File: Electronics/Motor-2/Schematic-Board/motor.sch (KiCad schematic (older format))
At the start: 42 parts, among them J1 CONN_02X05, J11 V, J12 U, J13 W, J2 RS485, J3 RS485, J4 CONN_01X06, J6 12, J9 GND, Q1 PSMN3R3-40YS, Q2 PSMN3R3-40YS, Q3 PSMN3R3-40YS, Q4 PSMN3R3-40YS, Q5 PSMN3R3-40YS, Q6 PSMN3R3-40YS, U1 STSPIN32F0, U2 LTC2876, U3 MA700, Y1 8Mhz

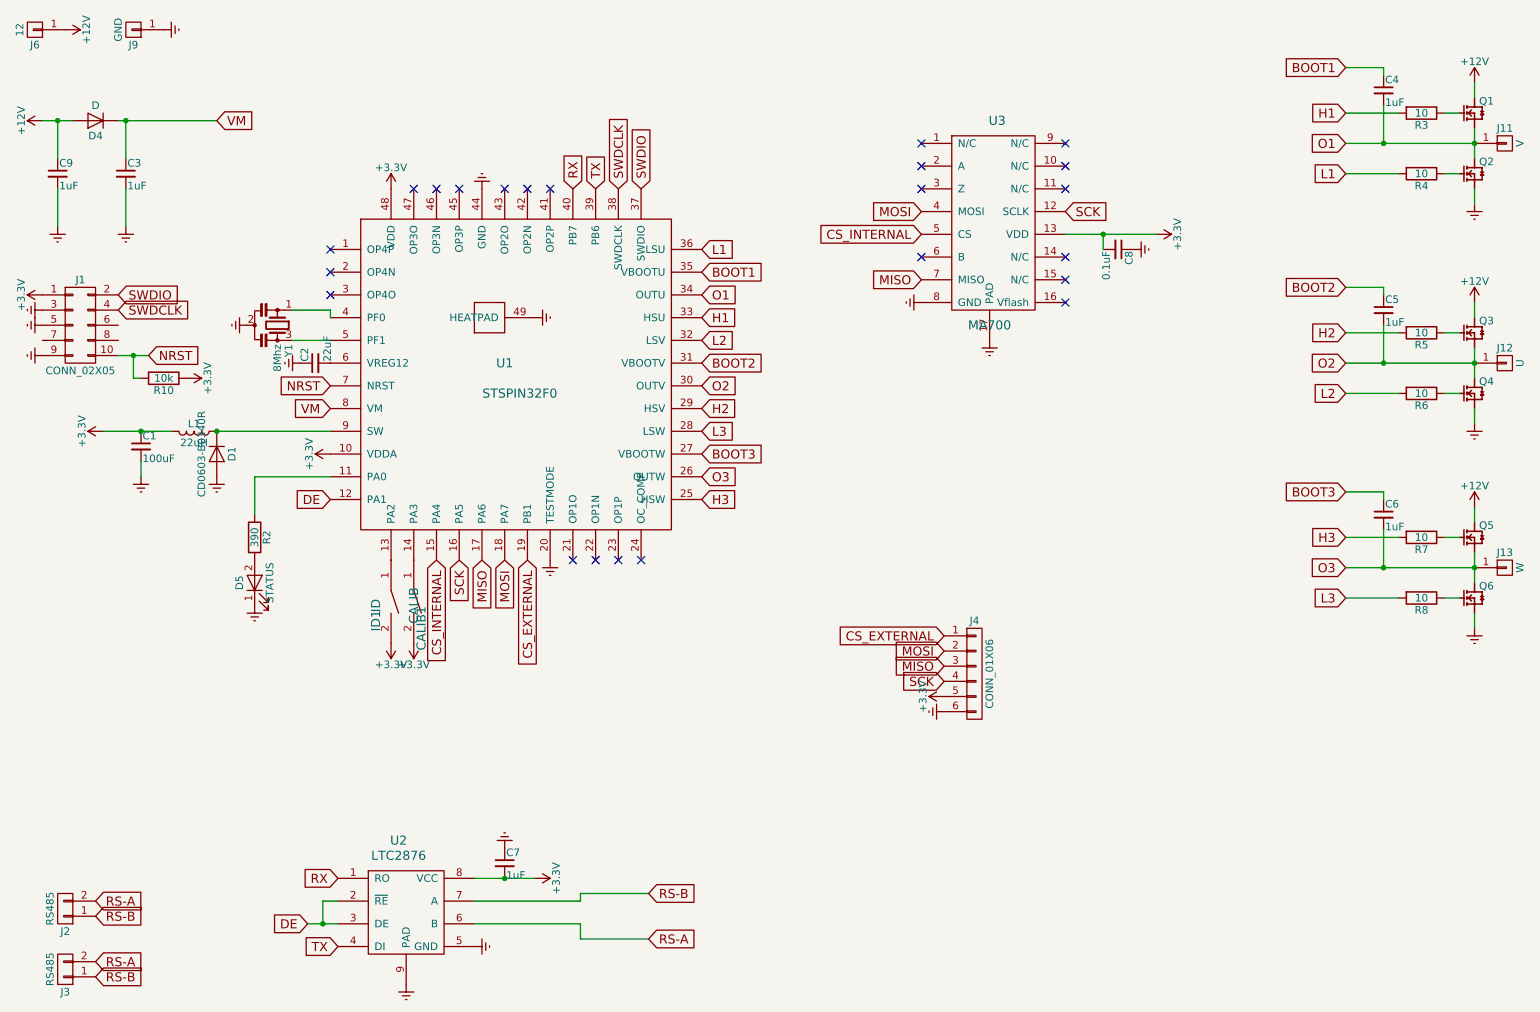
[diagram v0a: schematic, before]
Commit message: current changes
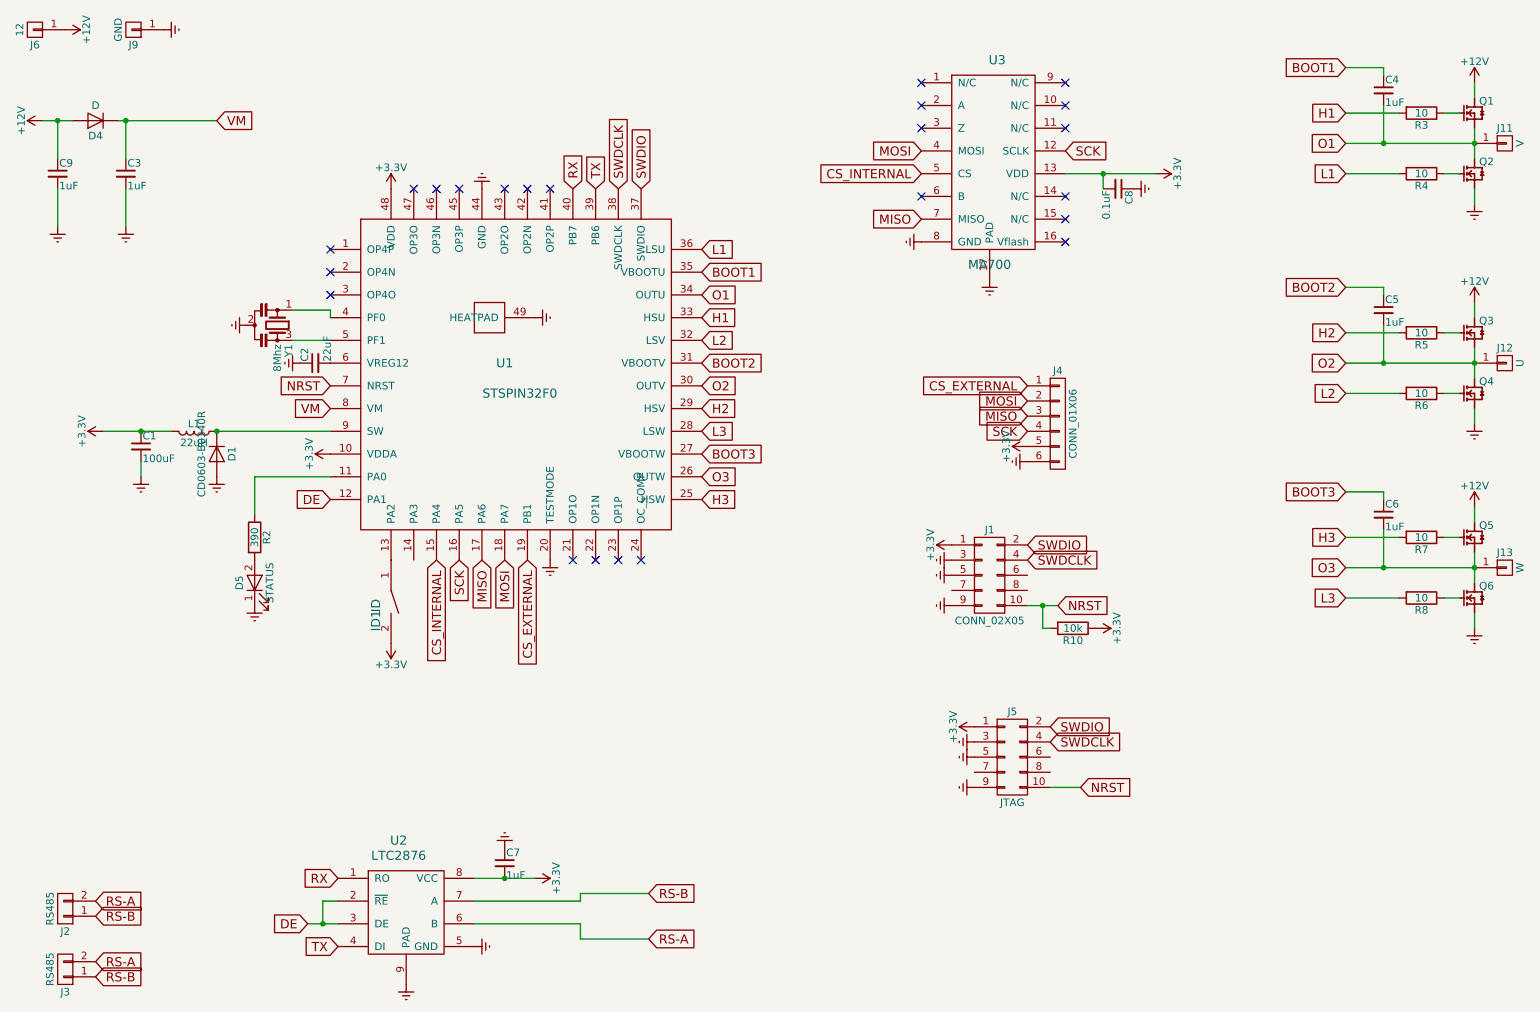
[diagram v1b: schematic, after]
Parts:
- removed CALIB1: CALIB, Resistors_SMD:R_1206, symbol B3U-1000P
- added J5: JTAG, Connectors:Tag-Connect_TC2050-IDC-NL, symbol CONN_02X05
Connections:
- net +3V3: now also J5.1 (P1)
- net Earth: now also J5.3 (P3), J5.5 (P5), J5.9 (P9)
- net NRST: now also J5.10 (P10)
- net SWDCLK: now also J5.4 (P4)
- net SWDIO: now also J5.2 (P2)
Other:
- moved on the sheet: C8, J1, J4, R10, U3
